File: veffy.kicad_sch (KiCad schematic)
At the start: 145 parts, among them CN1 XH-2AW_C2908611, J1 SWD, J2 Conn_Coaxial, J3 USB_C_Receptacle_USB2.0_14P, Q1 2N7002, Q2 BFR93A, Q3 2N7002, Q4 BFR93AE6327HTSA1, SW1 SW_Push, SW2 SW_Push, U1 ATSAMD21G18A-A, U10 MC34063AD, U11 AP2112K-3.3, U2 ADF4112BCPZ, U3 SA612AN/01_112, U4 MC3361, U5 LM386, U6 LM358_DFN, U7 AD9834, U8 QPA9510, U9 MCP73831-2-OT, Y2 C7527392

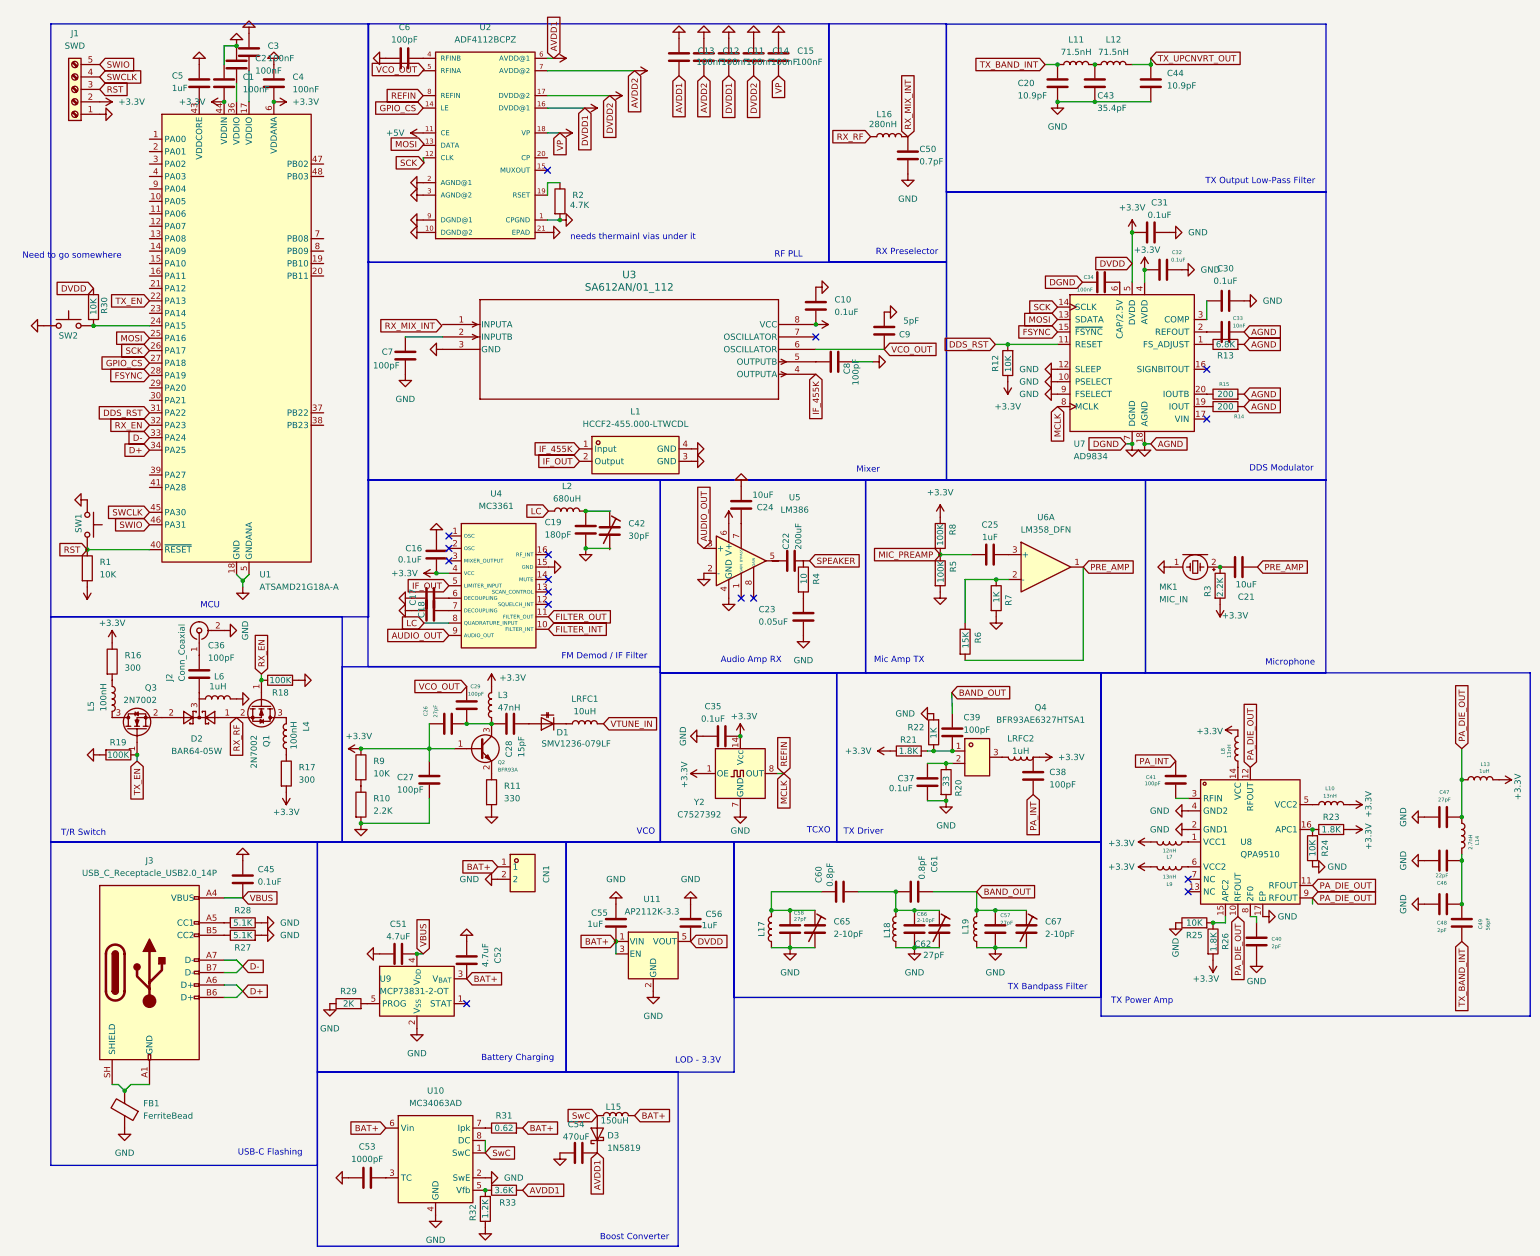
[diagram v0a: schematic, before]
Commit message: schematic fixes
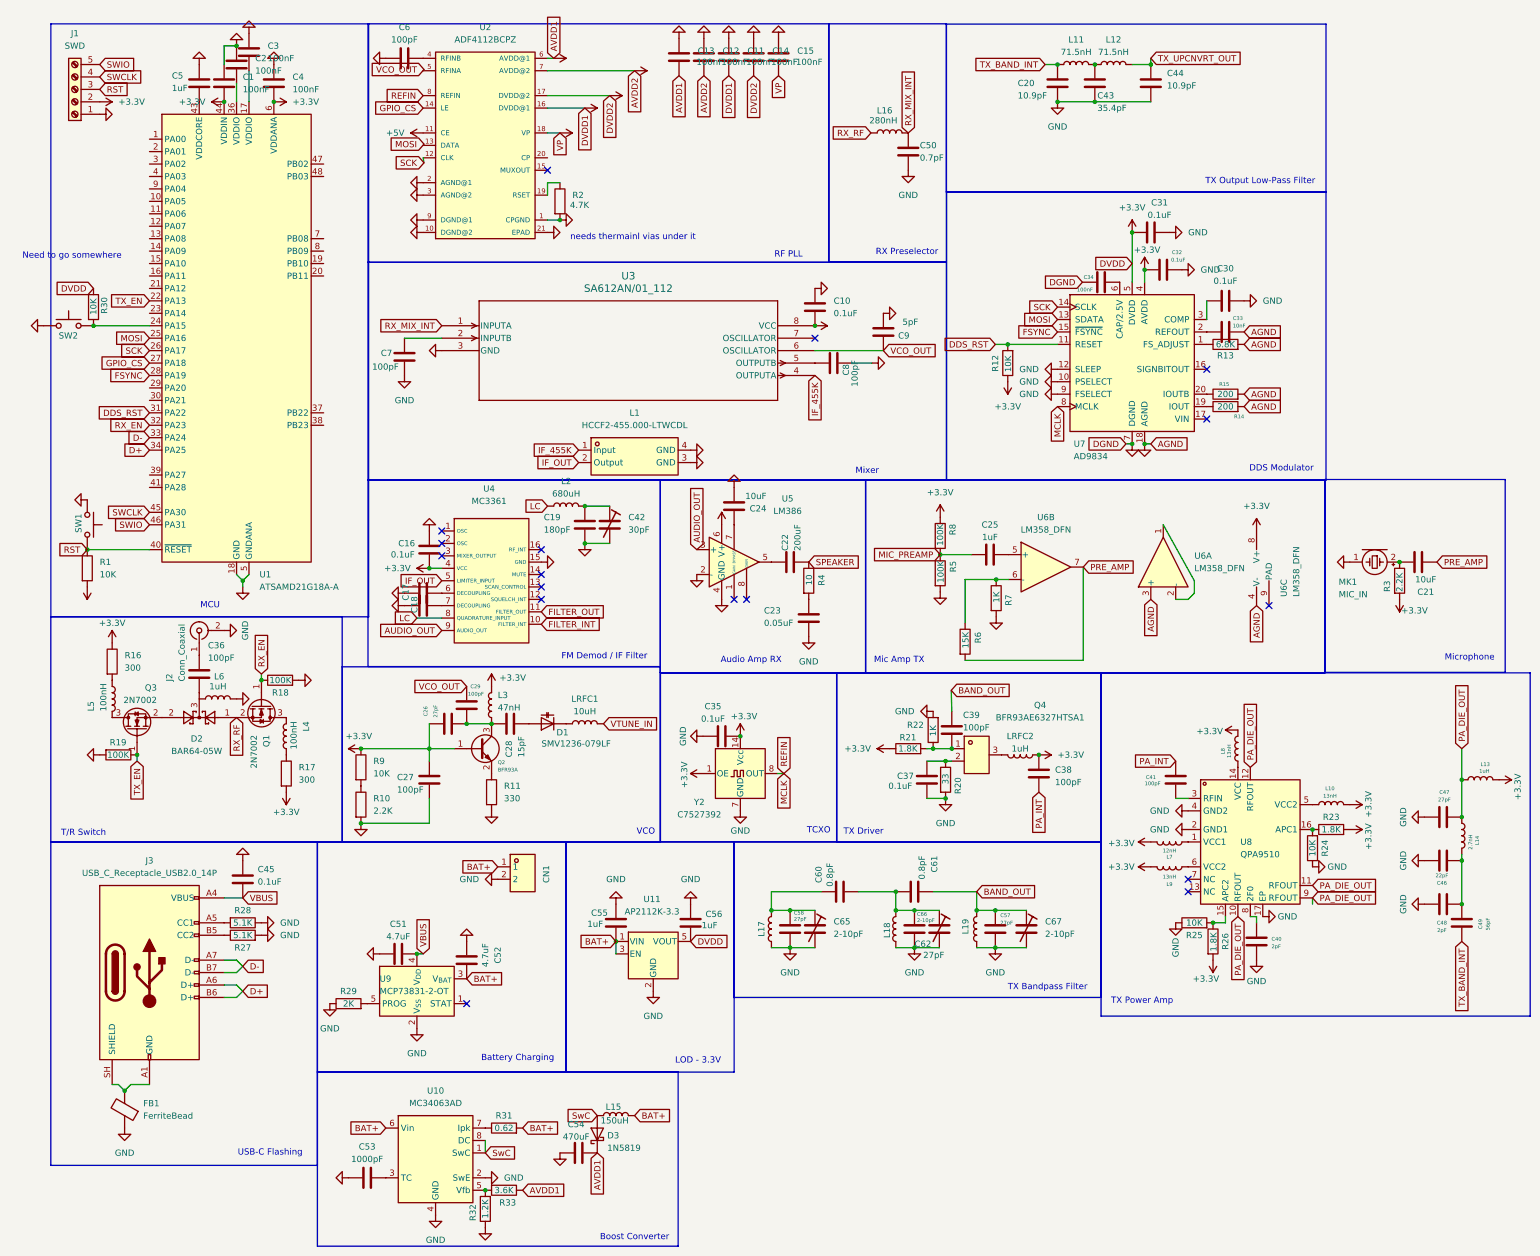
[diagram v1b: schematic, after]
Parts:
- added unit 1 of U6
- added unit 3 of U6
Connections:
- net +3.3V: now also C38.1, U6.8 (V+)
- net GND: now also C42.2, U6.3 (+), U6.4 (V-)
- net PRE_AMP: now also U6.7; no longer U6.1
- net RX_MIX_INT: now also U3.1 (INPUTA)
- net SPEAKER: now also R4.1
- net at R6.1, R7.1: now also U6.6 (-); no longer U6.2 (-)
- net at C19.1, L2.2: now also C42.1
- net at C25.2: now also U6.5 (+); no longer U6.3 (+)
- net at C22.1: now also U5.5
- new net: U6.1, U6.2 (-)
- no-connect marks 16 -> 17
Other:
- moved on the sheet: C16, C17, C18, C19, C23, C24, C38, C50, L16, L2, R4, U4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
